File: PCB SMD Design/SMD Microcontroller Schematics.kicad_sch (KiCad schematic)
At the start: 51 parts, among them J1 Power (9v), J10 Micro_SD_Card, J11 Throttle HallEffect, J12 Screen Connector, J13 Button 1, J14 Button 2, J15 Button 3, J16 Button 4, J17 Power OUT (9v), J18 Data (RX TX), J19 Power (9v), J2 Data (RX TX), J20 HC12, J21 Rotary SW, J3 Current Sensor, J4 Bat 1V, J5 Bat 1+2 V, J6 RPM Sensor, J7 Motor Temp, J8 Motor Controller Temp, J9 Motor Controller, U1 ESP32-DEVKIT-V1, U2 MCP6002-xP, U3 ADS1115IDGS, U4 ADS1115IDGS, U5 PC817, U6 ESP32-DEVKIT-V1

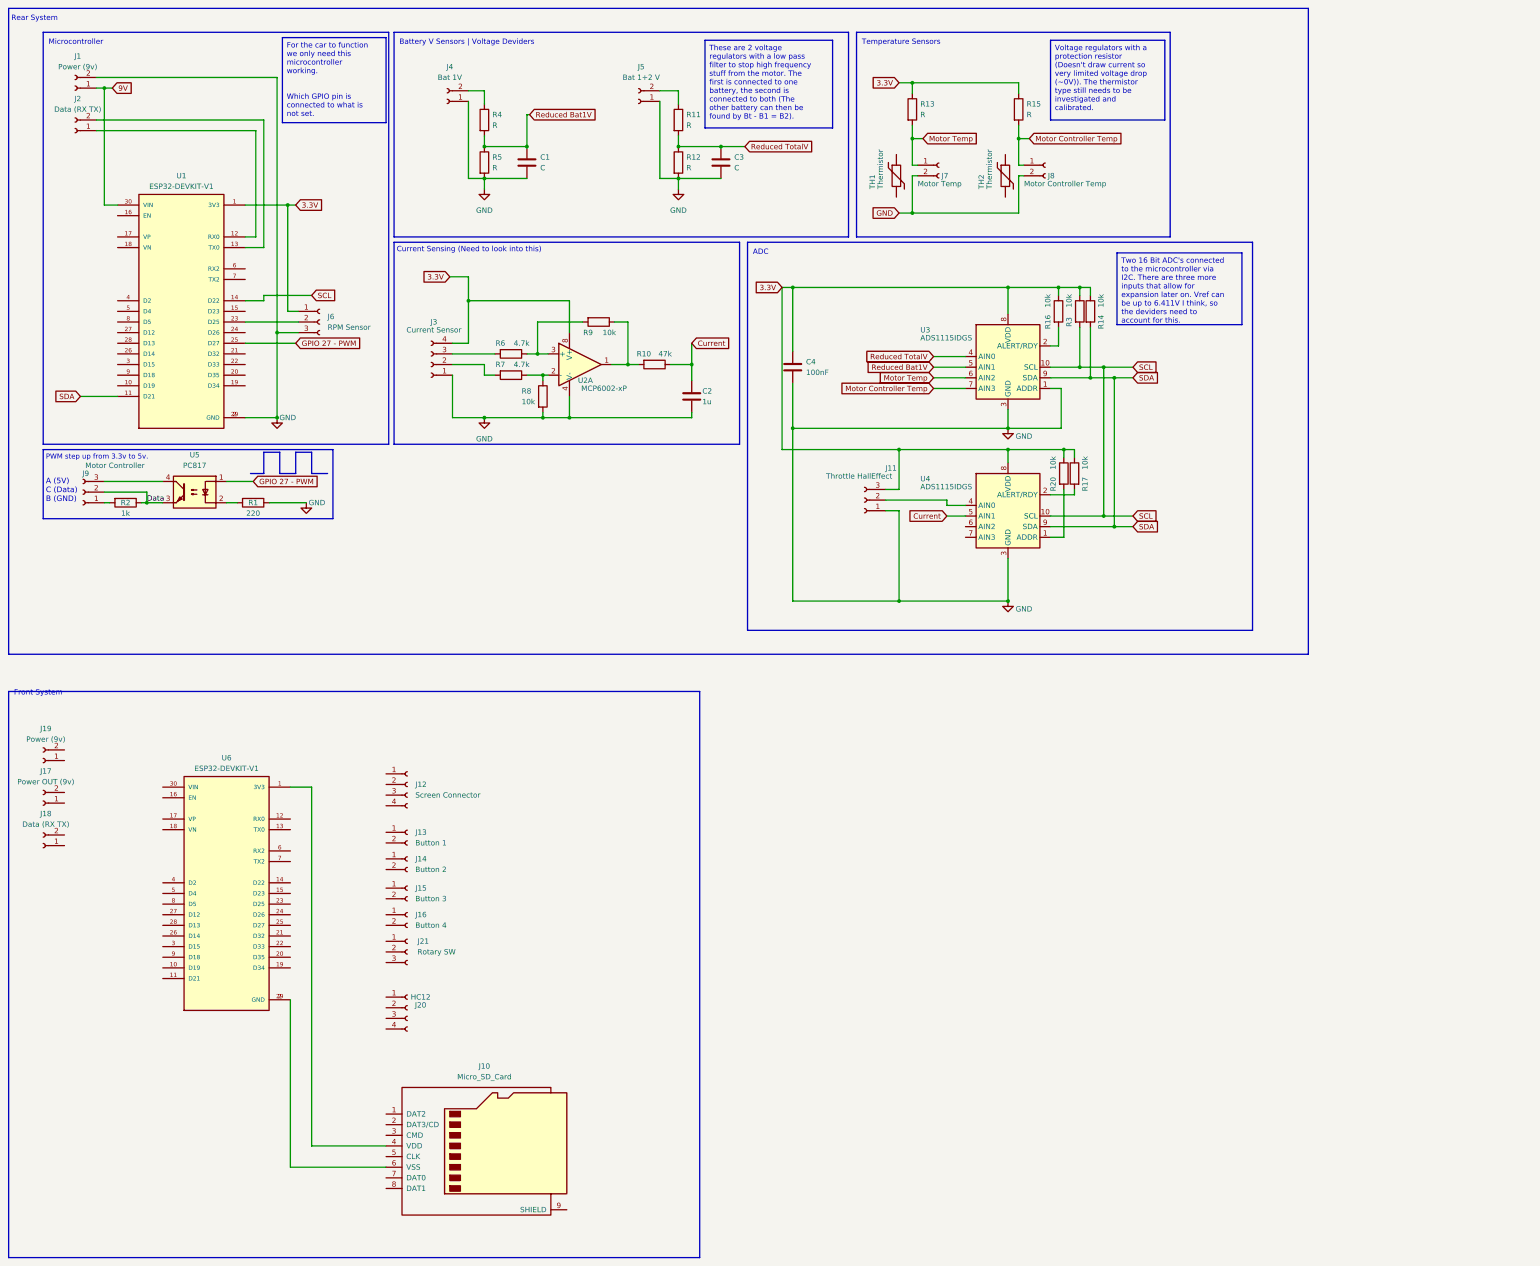
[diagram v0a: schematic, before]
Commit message: Many Changes
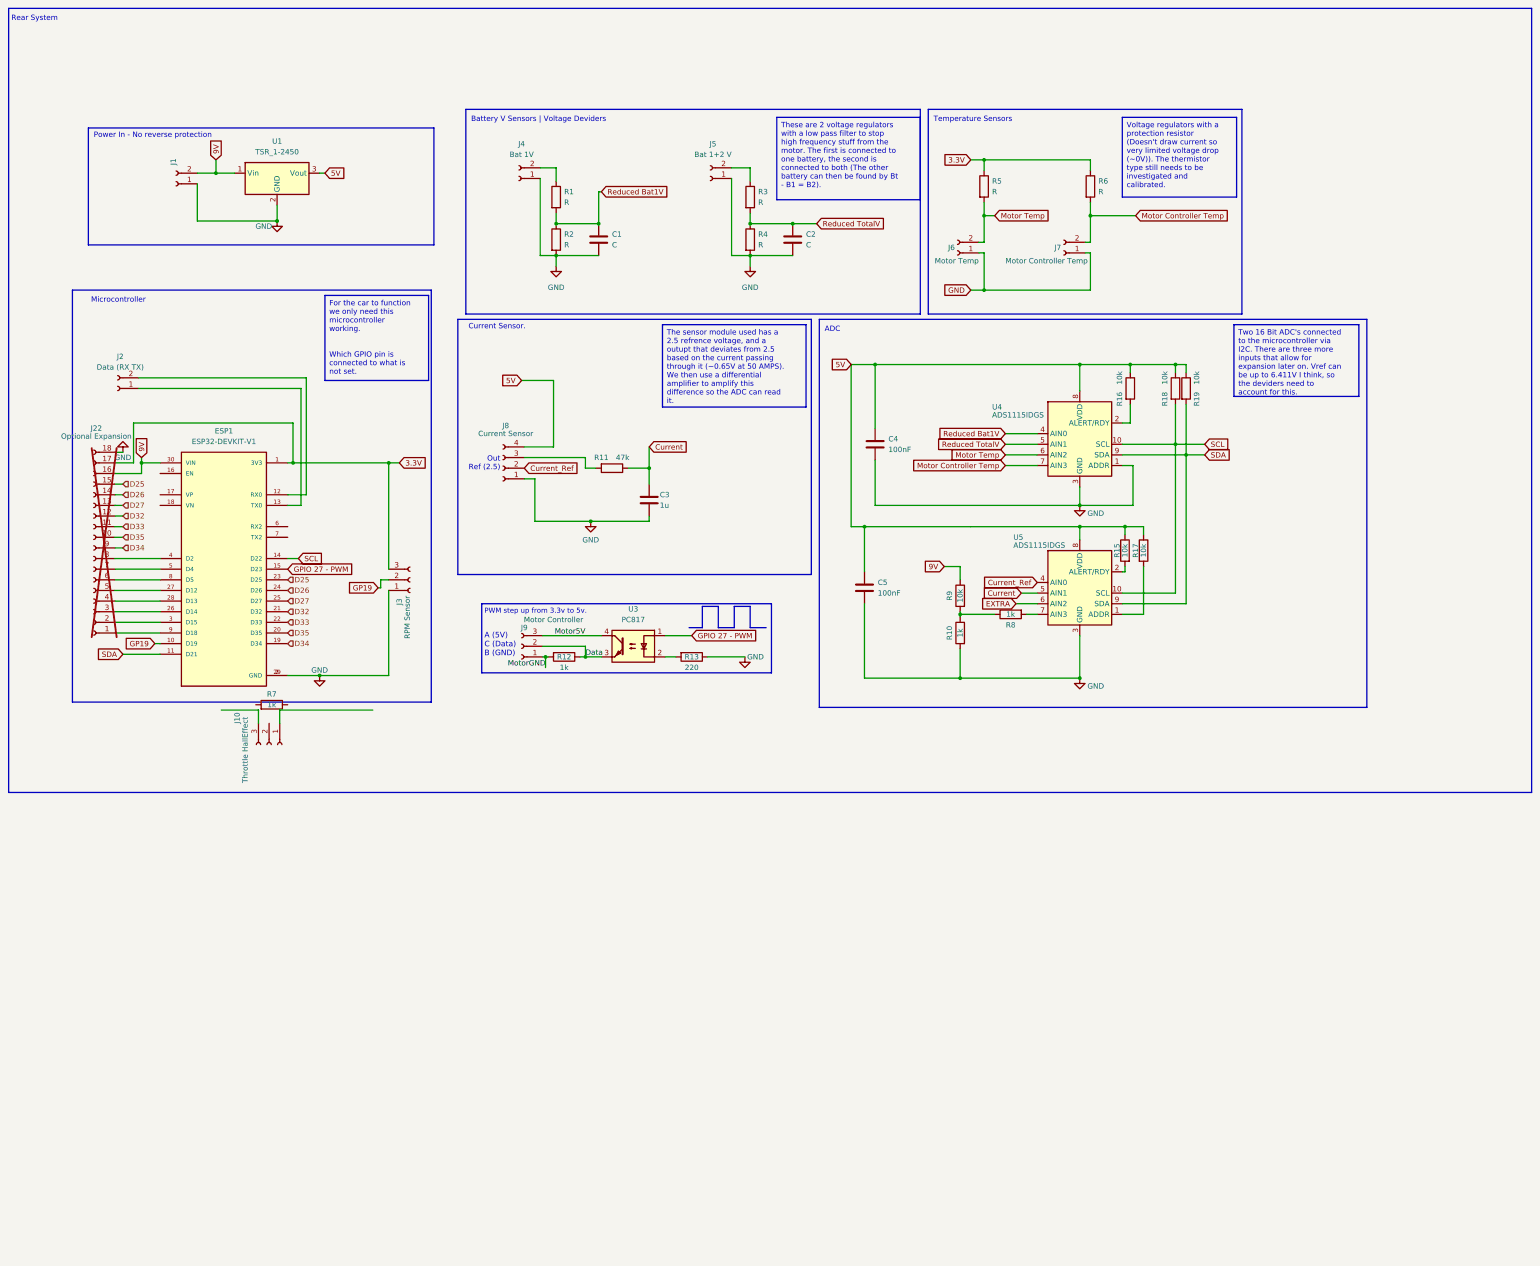
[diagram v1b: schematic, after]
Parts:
- removed J10: Micro_SD_Card, Connector_Card:microSD_HC_Hirose_DM3AT-SF-PEJM5, symbol Connector:Micro_SD_Card
- removed J11: Throttle HallEffect, Connector_PinHeader_2.54mm:PinHeader_1x03_P2.54mm_Horizontal, symbol Connector:Conn_01x03_Socket
- removed J12: Screen Connector, Connector_PinHeader_2.54mm:PinHeader_1x04_P2.54mm_Horizontal, symbol Connector:Conn_01x04_Socket
- removed J13: Button 1, Connector_PinHeader_2.54mm:PinHeader_1x02_P2.54mm_Horizontal, symbol Connector:Conn_01x02_Socket
- removed J14: Button 2, Connector_PinHeader_2.54mm:PinHeader_1x02_P2.54mm_Horizontal, symbol Connector:Conn_01x02_Socket
- removed J15: Button 3, Connector_PinHeader_2.54mm:PinHeader_1x02_P2.54mm_Horizontal, symbol Connector:Conn_01x02_Socket
- removed J16: Button 4, Connector_PinHeader_2.54mm:PinHeader_1x02_P2.54mm_Horizontal, symbol Connector:Conn_01x02_Socket
- removed J17: Power OUT (9v), Connector_PinHeader_2.54mm:PinHeader_1x02_P2.54mm_Horizontal, symbol Connector:Conn_01x02_Socket
- removed J18: Data (RX TX), Connector_PinHeader_2.54mm:PinHeader_1x02_P2.54mm_Horizontal, symbol Connector:Conn_01x02_Socket
- removed J19: Power (9v), Connector_PinHeader_2.54mm:PinHeader_1x02_P2.54mm_Horizontal, symbol Connector:Conn_01x02_Socket
- removed J20: HC12, Connector_PinHeader_2.54mm:PinHeader_1x04_P2.54mm_Horizontal, symbol Connector:Conn_01x04_Socket
- removed J21: Rotary SW, Connector_PinHeader_2.54mm:PinHeader_1x03_P2.54mm_Horizontal, symbol Connector:Conn_01x03_Socket
- removed J8: Motor Controller Temp, Connector_PinHeader_2.54mm:PinHeader_1x02_P2.54mm_Horizontal, symbol Connector:Conn_01x02_Socket
- removed R6: 4.7k, Resistor_SMD:R_1206_3216Metric, symbol Device:R
- removed TH1, TH2: Thermistor, symbol Device:Thermistor
- removed U2: MCP6002-xP, Package_DIP:DIP-8_W7.62mm_LongPads, symbol Amplifier_Operational:MCP6002-xP
- removed U6: ESP32-DEVKIT-V1, ESP32-DEVKIT-V1:MODULE_ESP32_DEVKIT_V1, symbol ESP32-DEVKIT-V1:ESP32-DEVKIT-V1
- added C5: 100nF, Capacitor_SMD:C_0805_2012Metric, symbol Device:C
- added J10: Throttle HallEffect, Connector_JST:JST_XH_B3B-XH-A_1x03_P2.50mm_Vertical, symbol Connector:Conn_01x03_Socket
- added J22: Optional Expansion, Connector_PinSocket_2.54mm:PinSocket_2x08_P2.54mm_Vertical, symbol Connector:Conn_01x18_Socket
- added J6: Motor Temp, Connector_JST:JST_XH_B2B-XH-A_1x02_P2.50mm_Vertical, symbol Connector:Conn_01x02_Socket
- added R10: 1k, Resistor_SMD:R_0805_2012Metric, symbol Device:R
- added U1: TSR_1-2450, Converter_DCDC:Converter_DCDC_TRACO_TSR-1_THT, symbol Regulator_Switching:TSR_1-2450
- C1, C4: footprint Capacitor_SMD:C_1206_3216Metric -> Capacitor_SMD:C_0805_2012Metric
- C2: renamed from C3; footprint Capacitor_SMD:C_1206_3216Metric -> Capacitor_SMD:C_0805_2012Metric
- C3: renamed from C2; footprint Capacitor_SMD:C_1206_3216Metric -> Capacitor_SMD:C_0805_2012Metric
- ESP1: renamed from U1; now left out of the parts list
- J1, J2: footprint Connector_PinHeader_2.54mm:PinHeader_1x02_P2.54mm_Horizontal -> Connector_JST:JST_XH_B2B-XH-A_1x02_P2.50mm_Vertical
- J3: renamed from J6; footprint Connector_PinSocket_2.54mm:PinSocket_1x03_P2.54mm_Horizontal -> Connector_JST:JST_XH_B3B-XH-A_1x03_P2.50mm_Vertical
- J4, J5: footprint Connector_PinHeader_2.54mm:PinHeader_1x02_P2.54mm_Horizontal -> Connector_JST:JST_XH_B2B-XH-A_1x02_P2.50mm_Vertical; now left out of the parts list
- J7: value Motor Temp -> Motor Controller Temp; footprint Connector_PinHeader_2.54mm:PinHeader_1x02_P2.54mm_Horizontal -> Connector_JST:JST_XH_B2B-XH-A_1x02_P2.50mm_Vertical; now left out of the parts list
- J8: renamed from J3; footprint Connector_PinHeader_2.54mm:PinHeader_1x04_P2.54mm_Horizontal -> Connector_JST:JST_XH_B4B-XH-A_1x04_P2.50mm_Vertical
- J9: footprint Connector_PinHeader_2.54mm:PinHeader_1x03_P2.54mm_Horizontal -> Connector_JST:JST_XH_B3B-XH-A_1x03_P2.50mm_Vertical
- R1: renamed from R4; footprint Resistor_SMD:R_1206_3216Metric -> Resistor_SMD:R_0805_2012Metric
- R11: renamed from R10; footprint Resistor_SMD:R_1206_3216Metric -> Resistor_SMD:R_0805_2012Metric
- R12: renamed from R2; footprint Resistor_SMD:R_1206_3216Metric -> Resistor_SMD:R_0805_2012Metric
- R13: renamed from R1; footprint Resistor_SMD:R_1206_3216Metric -> Resistor_SMD:R_0805_2012Metric
- R15: renamed from R17; footprint Resistor_SMD:R_1206_3216Metric -> Resistor_SMD:R_0805_2012Metric
- R16, R9: footprint Resistor_SMD:R_1206_3216Metric -> Resistor_SMD:R_0805_2012Metric
- R17: renamed from R20; footprint Resistor_SMD:R_1206_3216Metric -> Resistor_SMD:R_0805_2012Metric
- R18: renamed from R3; footprint Resistor_SMD:R_1206_3216Metric -> Resistor_SMD:R_0805_2012Metric
- R19: renamed from R14; footprint Resistor_SMD:R_1206_3216Metric -> Resistor_SMD:R_0805_2012Metric
- R2: renamed from R5; footprint Resistor_SMD:R_1206_3216Metric -> Resistor_SMD:R_0805_2012Metric
- R3: renamed from R11; footprint Resistor_SMD:R_1206_3216Metric -> Resistor_SMD:R_0805_2012Metric
- R4: renamed from R12; footprint Resistor_SMD:R_1206_3216Metric -> Resistor_SMD:R_0805_2012Metric
- R5: renamed from R13; footprint Resistor_SMD:R_1206_3216Metric -> Resistor_SMD:R_0805_2012Metric
- R6: renamed from R15; footprint Resistor_SMD:R_1206_3216Metric -> Resistor_SMD:R_0805_2012Metric
- R7: value 4.7k -> 1k; footprint Resistor_SMD:R_1206_3216Metric -> Resistor_SMD:R_0805_2012Metric
- R8: value 10k -> 1k; footprint Resistor_SMD:R_1206_3216Metric -> Resistor_SMD:R_0805_2012Metric
- U3: renamed from U5; now left out of the parts list
- renumbered U3 to U4, U4 to U5
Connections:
- net 3.3V: now also J3.3 (Pin_3), J22.17 (Pin_17); no longer C4.1, J3.1 (Pin_1), J8.4 (Pin_4), R15.1, R16.1, R17.1, R18.1, R19.1, U4.8 (VDD), U5.8 (VDD)
- net 9V: now also J1.2 (Pin_2), R9.1, J22.16 (Pin_16), U1.1 (Vin); no longer J1.1 (Pin_1)
- net GND: now also J1.1 (Pin_1), J3.1 (Pin_1), J7.1 (Pin_1), C5.2, J22.18 (Pin_18), J6.1 (Pin_1), R10.2, U1.2 (GND); no longer J1.2 (Pin_2), J3.3 (Pin_3), J7.2 (Pin_2), R8.2
- net GPIO 27 - PWM: now also ESP1.15 (D23); no longer ESP1.25 (D27)
- net Motor Controller Temp: now also J7.2 (Pin_2)
- net Motor Temp: now also J6.2 (Pin_2); no longer J7.1 (Pin_1)
- net Reduced Bat1V: now also U4.4 (AIN0); no longer U4.5 (AIN1)
- net Reduced TotalV: now also U4.5 (AIN1); no longer U4.4 (AIN0)
- net Motor5V: now reaches J9.3 (Pin_3), U3.4
- net GP19: now reaches ESP1.10 (D19)
- net GP19: now also J3.2 (Pin_2)
- net at ESP1.12 (RX0): now also J2.2 (Pin_2); no longer J2.1 (Pin_1)
- net at ESP1.13 (TX0): now also J2.1 (Pin_1); no longer J2.2 (Pin_2)
- net D34: now reaches ESP1.19 (D34)
- net D34: now also J22.9 (Pin_9)
- net D35: now reaches ESP1.20 (D35)
- net D35: now also J22.10 (Pin_10)
- net D32: now reaches ESP1.21 (D32)
- net D32: now also J22.12 (Pin_12)
- net D33: now reaches ESP1.22 (D33)
- net D33: now also J22.11 (Pin_11)
- net D25: now reaches ESP1.23 (D25)
- net D25: now also J22.15 (Pin_15); no longer J3.2 (Pin_2)
- net D26: now reaches ESP1.24 (D26)
- net D26: now also J22.14 (Pin_14)
- net at ESP1.26 (D14): now also J22.3 (Pin_3)
- net at ESP1.27 (D12): now also J22.5 (Pin_5)
- net at ESP1.28 (D13): now also J22.4 (Pin_4)
- net at ESP1.3 (D15): now also J22.2 (Pin_2)
- net at ESP1.4 (D2): now also J22.8 (Pin_8)
- net at ESP1.5 (D4): now also J22.7 (Pin_7)
- net at ESP1.8 (D5): now also J22.6 (Pin_6)
- net at ESP1.9 (D18): now also J22.1 (Pin_1)
- net Current_Ref: now reaches U5.4 (AIN0)
- net Current_Ref: now also J8.2 (Pin_2)
- net EXTRA: now reaches U5.6 (AIN2)
- net at U5.7 (AIN3): now also R8.2
- net at R7.2: no longer J8.2 (Pin_2)
- net at J8.3 (Pin_3): now also R11.2
- net MotorGND: now reaches J9.1 (Pin_1), R12.2
- net at R9.2: now also R8.1, R10.1
- net at R7.1: no longer R8.1
- new net 5V: C4.1, C5.1, J8.4 (Pin_4), R15.1, R16.1, R17.1, R18.1, R19.1, U1.3 (Vout), U4.8 (VDD), U5.8 (VDD)
- new net D27: ESP1.25 (D27), J22.13 (Pin_13)
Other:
- note added: "Current Sensor."
- note added: "Out Ref (2.5)"
- note added: "Power In - No reverse protection"
- note removed: "Current Sensing (Need to look into this)"
- note removed: "Front System"
- moved on the sheet: C1, C2, C3, C4, ESP1, J2, J3, J4, J5, J8, J9, R1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
